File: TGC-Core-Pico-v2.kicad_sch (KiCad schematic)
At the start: 36 parts, among them J2 Conn_01x18, J3 Conn_01x18, P1 USB_C_Plug_USB2.0, SW1 SW_Push, U1 RP2040, U2 AMS1117-3.3, U3 W25Q128JVS, U4 ESP32-C6-MINI-1, U5 SHT31-DIS, U6 ICM-20602, Y1 ABM8-272-T3

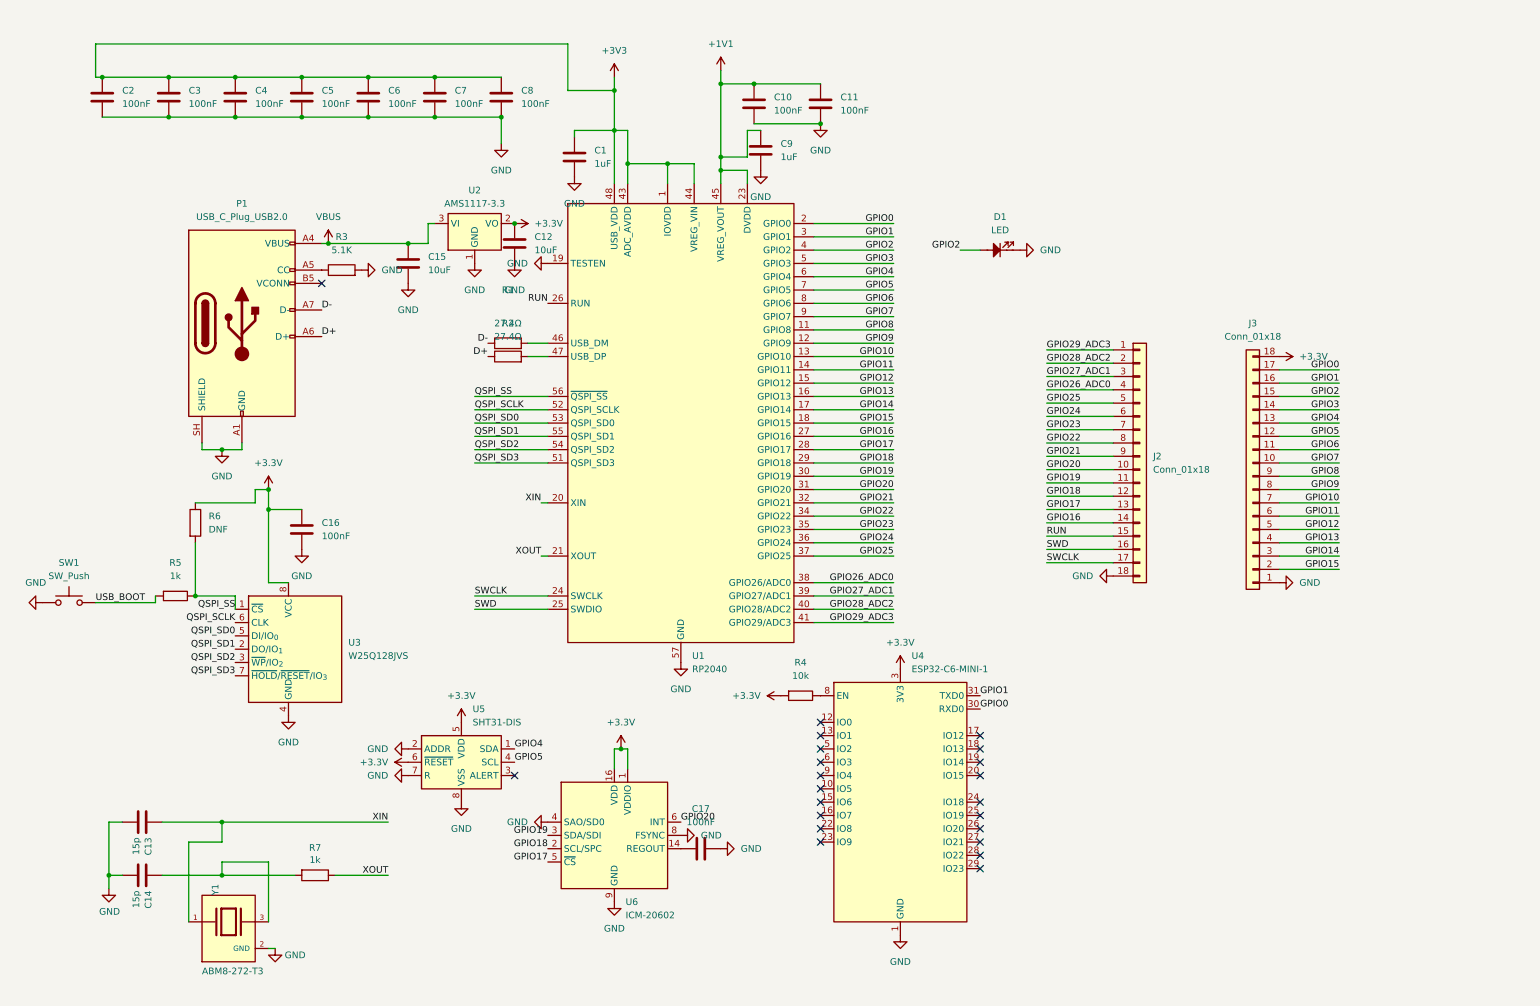
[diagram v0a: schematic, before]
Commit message: Add files via upload
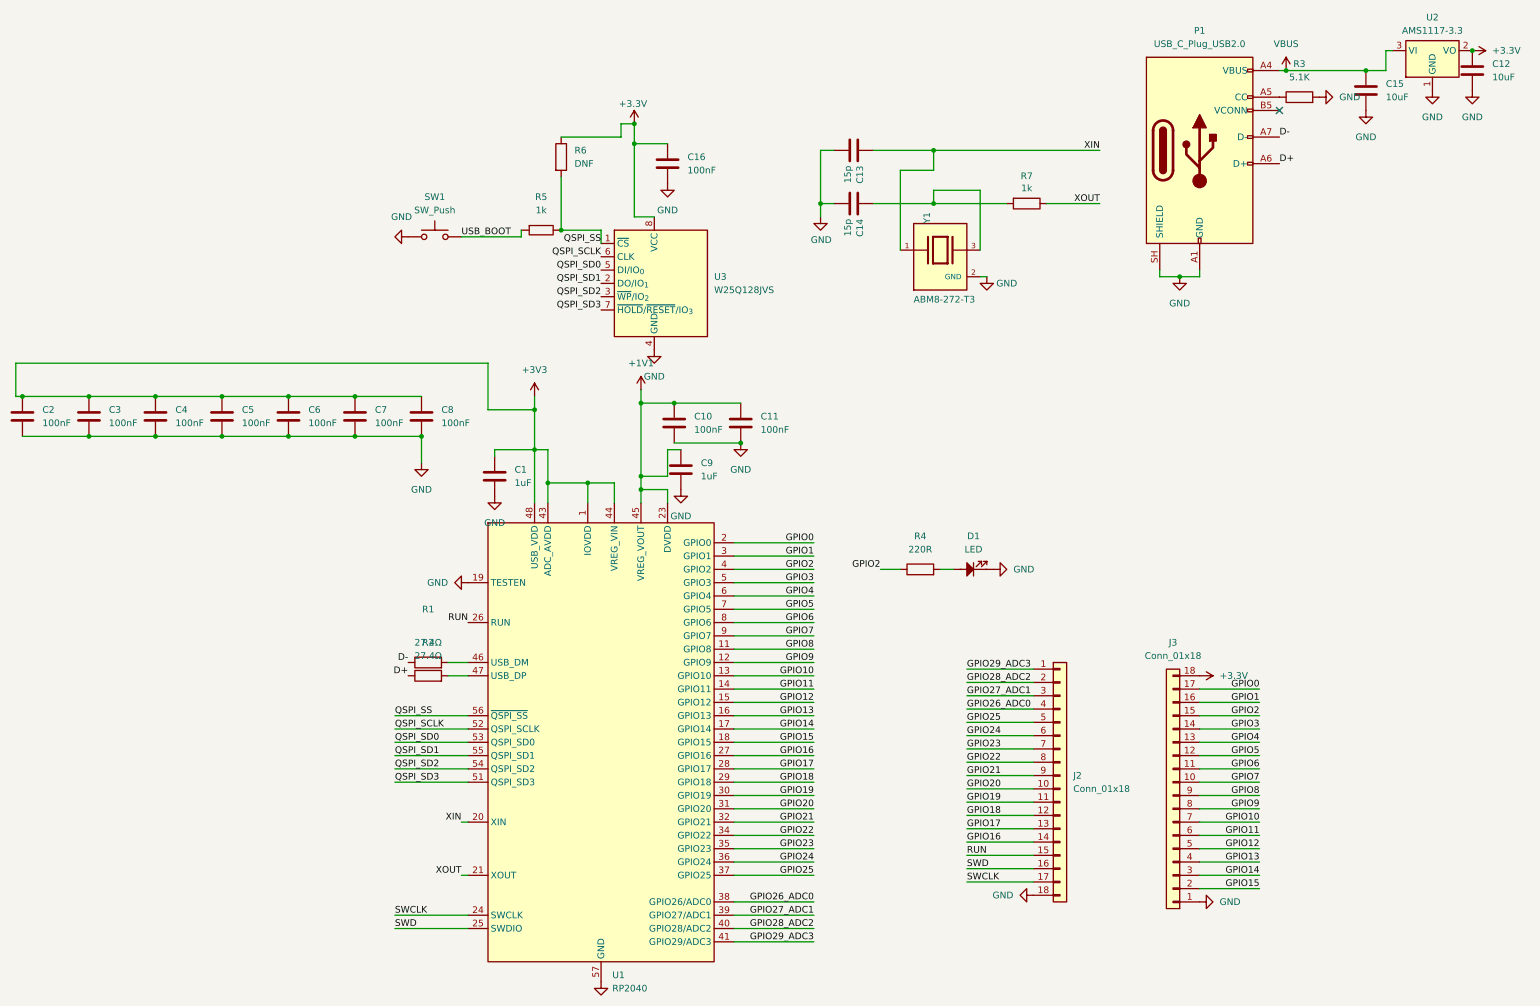
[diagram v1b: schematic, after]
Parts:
- removed C17: 100nF, Capacitor_SMD:C_0805_2012Metric, symbol Device:C
- removed R4: 10k, Resistor_SMD:R_0402_1005Metric, symbol PCM_SL_Resistors:10k
- removed U4: ESP32-C6-MINI-1, RF_Module:ESP32-C6-MINI-1, symbol RF_Module:ESP32-C6-MINI-1
- removed U5: SHT31-DIS, Sensor_Humidity:Sensirion_DFN-8-1EP_2.5x2.5mm_P0.5mm_EP1.1x1.7mm, symbol Sensor_Humidity:SHT31-DIS
- removed U6: ICM-20602, Package_LGA:LGA-16_3x3mm_P0.5mm_LayoutBorder3x5y, symbol Sensor_Motion:ICM-20602
- added R4: 220R, Resistor_SMD:R_0402_1005Metric, symbol Device:R
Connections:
- net GPIO2: now also R4.1; no longer D1.2
- new net: D1.2, R4.2
- no-connect marks 22 -> 1
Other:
- moved on the sheet: C1, C10, C11, C12, C13, C14, C15, C16, C2, C3, C4, C5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
